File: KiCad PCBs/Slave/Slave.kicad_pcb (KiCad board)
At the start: 2 copper layers, 83.8 x 71.1 mm, 48 parts, among them J1 Screw_Terminal_01x02, J10 AVR-ISP-6, J11 Conn_01x06_Female, J12 Screw_Terminal_01x02, J13 Screw_Terminal_01x02, J14 Screw_Terminal_01x02, J15 Screw_Terminal_01x02, J16 Screw_Terminal_01x02, J2 Screw_Terminal_01x02, J3 Screw_Terminal_01x02, J4 Screw_Terminal_01x02, J5 Screw_Terminal_01x02, J6 Screw_Terminal_01x02, J7 Screw_Terminal_01x02, J8 Screw_Terminal_01x02, J9 Screw_Terminal_01x02, SW1 SW_DIP_x02, SW2 SW_DIP_x02, SW3 SW_MEC_5E, U1 ATmega328P-AU, U2 MAX487ESA+T, U3 ULN2003A, U5 AMS1117-5.0, Y1 Crystal_GND24

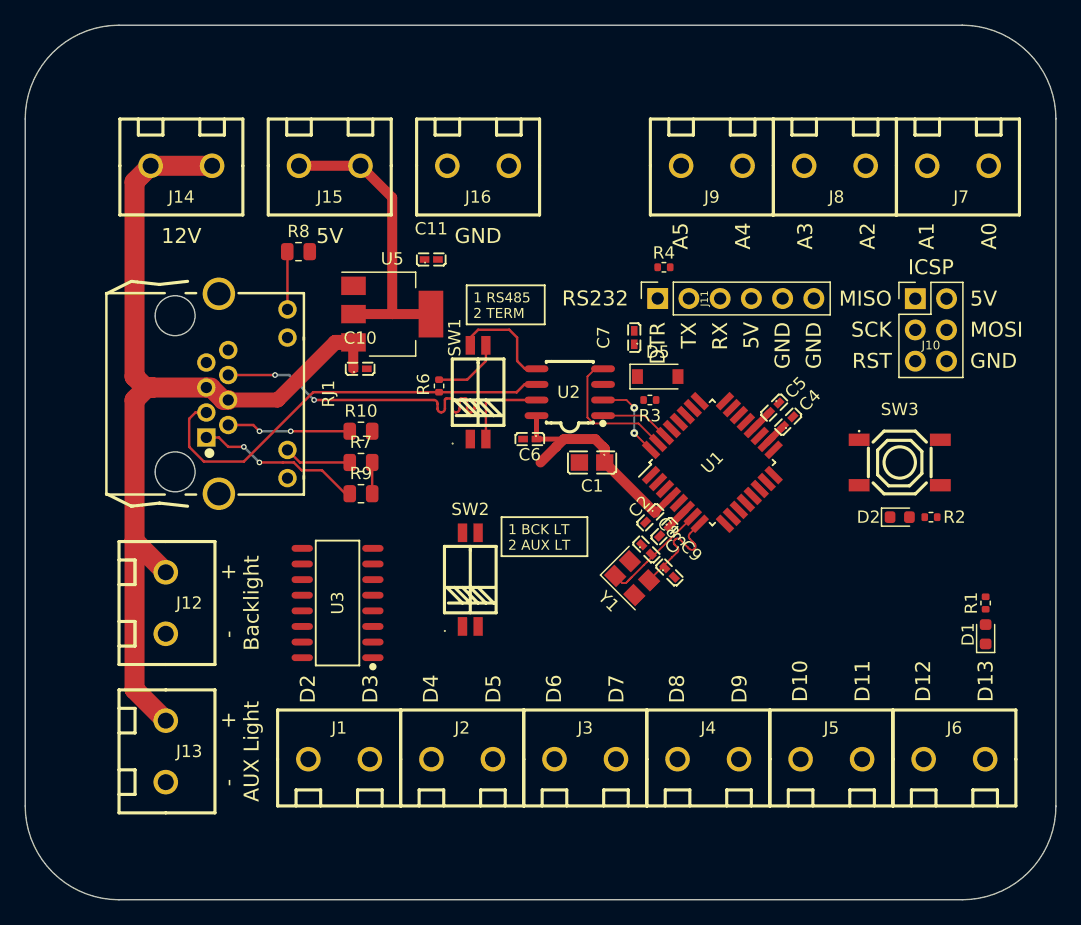
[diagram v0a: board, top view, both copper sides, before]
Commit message: Slave WIP
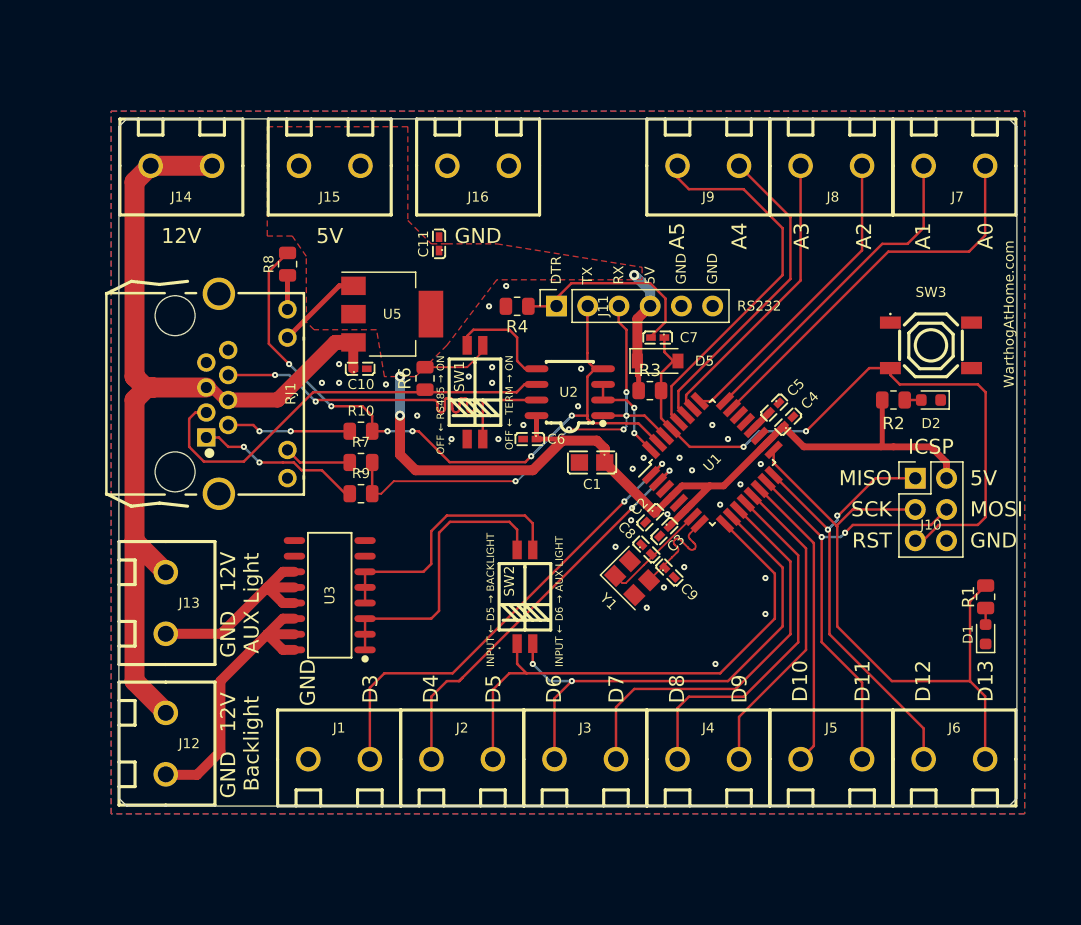
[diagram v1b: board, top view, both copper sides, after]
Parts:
- C8, C9: value 16pF -> 15pF
- R1, R2, R3, R4, R6: footprint Resistor_SMD:R_0402_1005Metric -> Resistor_SMD:R_0805_2012Metric
- moved J10 14.6 mm to (166.4, 105.4)
- moved R4 12.4 mm to (134.0, 91.4), turned to 180 degrees
- moved J13 12.1 mm to (105.4, 115.6)
- moved J12 11.4 mm to (105.4, 127.0)
- moved R2 10.0 mm to (164.6, 99.1), turned to 0 degrees
- moved SW3 9.86 mm to (167.6, 94.6)
- moved D2 9.86 mm to (167.6, 99.1), turned to 180 degrees
- moved J11 8.25 mm to (137.2, 91.4)
- moved SW2 4.66 mm to (134.6, 115.1)
- moved C7 1.91 mm to (145.4, 94.0), turned to 180 degrees
- moved C11 1.42 mm to (127.6, 86.4), turned to 90 degrees
- moved R8 1.35 mm to (115.3, 88.0), turned to 90 degrees
- moved R6 1.30 mm to (126.5, 97.3)
- moved D5 1.27 mm to (145.4, 95.9)
- moved U3 0.90 mm to (118.7, 114.9)
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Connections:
- J1 pad 1: D2 -> GND
- R1 pad 1: D13/SCK -> D13
- SW2 pad 1: D3 -> D5
- SW2 pad 2: D4 -> D6
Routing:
- net RESET: track 0.00 -> 55.5 mm, vias 0 -> 2
- net D13: track 0.00 -> 51.2 mm
- net TXD: track 11.5 -> 57.1 mm, vias 0 -> 6
- net D5: track 0.00 -> 43.1 mm
- net D6: track 0.00 -> 41.9 mm, vias 0 -> 2
- net D3: track 0.00 -> 38.4 mm, vias 0 -> 2
- net D12: track 0.00 -> 37.2 mm, vias 0 -> 2
- net D11: track 0.00 -> 36.8 mm, vias 0 -> 2
- net +5V: track 47.6 -> 83.8 mm, vias 0 -> 3
- net D4: track 0.00 -> 33.8 mm, vias 0 -> 2
- net D7: track 0.00 -> 32.7 mm
- net RXD: track 8.26 -> 40.6 mm, vias 0 -> 5
- net A0: track 0.00 -> 32.1 mm
- net A5: track 0.00 -> 31.0 mm
- net D8: track 0.00 -> 29.3 mm
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- added copper zone on F.Cu, net +5V
- added copper zone on B.Cu, net GND
- added copper zone on F.Cu, net GND
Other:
- board size 83.8 x 71.1 mm -> 73 x 55.9 mm
- board text added: "GND"
- board text added: "INPUT ← D5 → BACKLIGHT"
- board text added: "INPUT ← D6 → AUX LIGHT"
- board text added: "OFF ← RS485 → ON"
- board text added: "OFF ← TERM → ON"
- board text added: "WarthogAtHome.com"
- board text removed: "1 BCK LT"
- board text removed: "1 RS485"
- board text removed: "2 AUX LT"
- board text removed: "2 TERM"
